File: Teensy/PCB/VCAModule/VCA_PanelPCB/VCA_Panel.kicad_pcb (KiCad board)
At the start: 2 copper layers, 55.9 x 128 mm, 21 parts

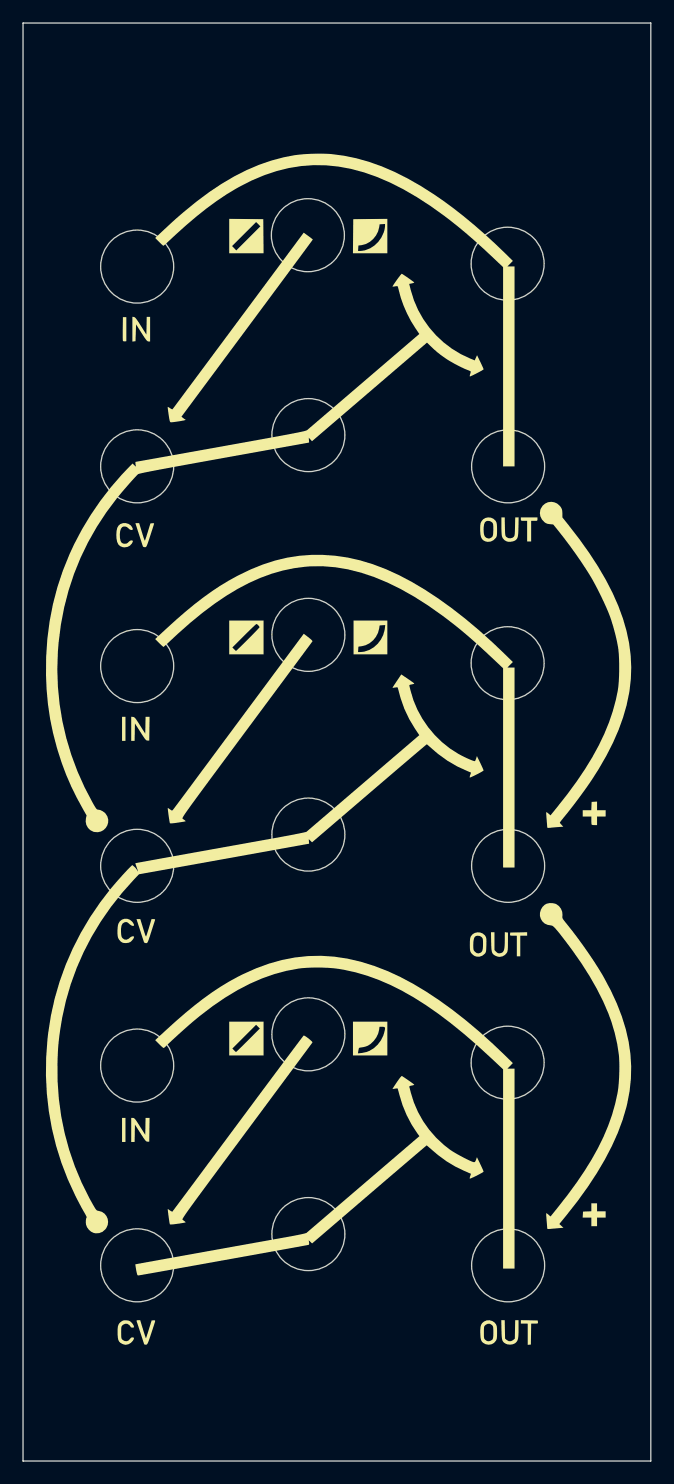
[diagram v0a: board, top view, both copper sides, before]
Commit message: Generated Gerbers
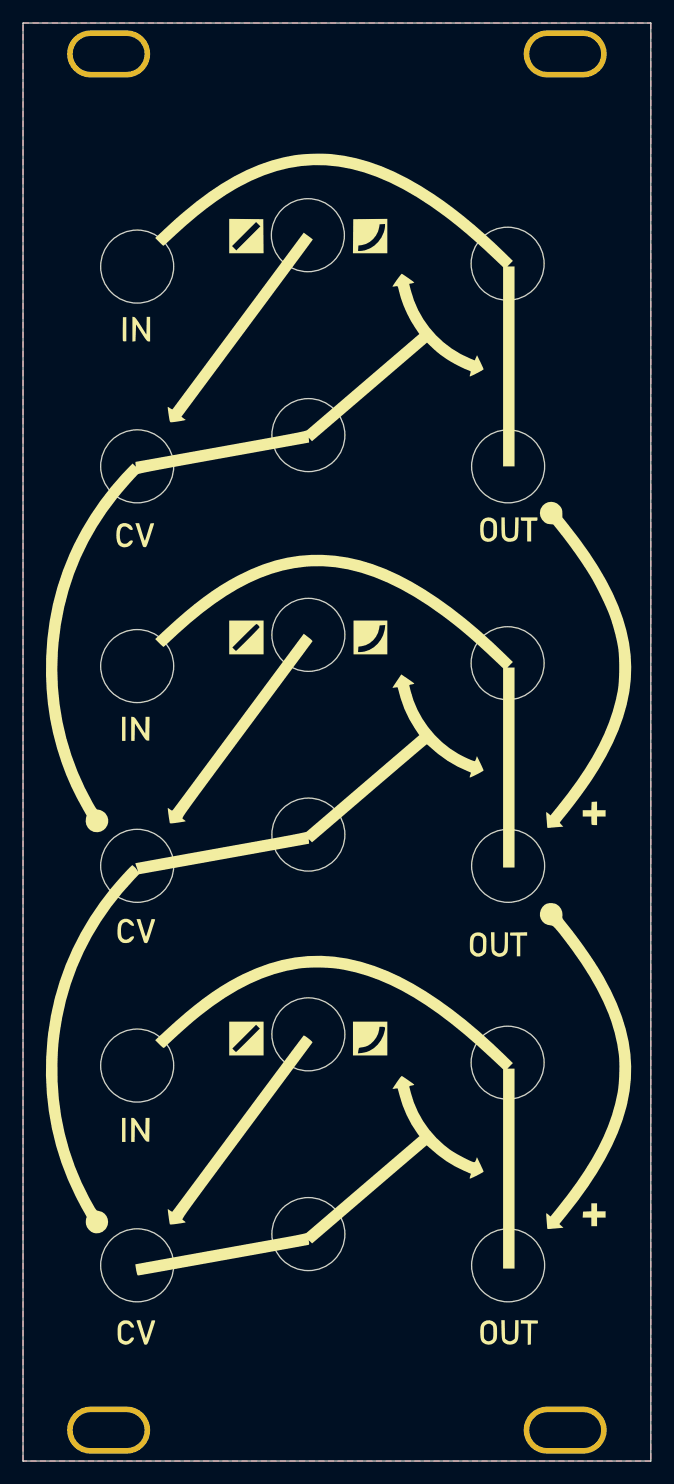
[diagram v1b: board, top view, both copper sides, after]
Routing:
- added copper zone on B.Cu, net shielding
- added copper zone on F.Cu, net shielding
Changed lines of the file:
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@@
       (layerselection 0x00010fc_ffffffff)
       (disableapertmacros false)
-      (usegerberextensions false)
-      (usegerberattributes true)
-      (usegerberadvancedattributes true)
-      (creategerberjobfile true)
+      (usegerberextensions true)
+      (usegerberattributes false)
+      (usegerberadvancedattributes false)
+      (creategerberjobfile false)
       (svguseinch false)
       (svgprecision 6)
@@
       (psa4output false)
       (plotreference true)
-      (plotvalue true)
+      (plotvalue false)
       (plotinvisibletext false)
       (sketchpadsonfab false)
-      (subtractmaskfromsilk false)
+      (subtractmaskfromsilk true)
       (outputformat 1)
       (mirror false)
-      (drillshape 1)
+      (drillshape 0)
       (scaleselection 1)
-      (outputdirectory "")
+      (outputdirectory "VCA_Panel_Gerber")
     )
   )
   (net 0 "")
+  (net 1 "shielding")
   (footprint "Perfboard:3.5mm Jack Perfboard_Hole" (layer "F.Cu")
     (at 114.3 160.02)
@@
     (fp_line (start -2.54 -64) (end 2.54 -64) (layer "User.1") (width 0.12))
     (fp_circle (center 0 0) (end 0 0) (layer "User.1") (width 0.12) (fill none))
-    (fp_line (start -1.27 59.65) (end 1.27 59.65) (layer "User.2") (width 0.12))
-    (fp_line (start -1.27 62.85) (end 1.27 62.85) (layer "User.2") (width 0.12))
-    (fp_line (start -1.27 -62.85) (end 1.27 -62.85) (layer "User.2") (width 0.12))
-    (fp_line (start -1.27 -59.65) (end 1.27 -59.65) (layer "User.2") (width 0.12))
-    (fp_arc (start 1.27 -62.85) (mid 2.87 -61.25) (end 1.27 -59.65) (layer "User.2") (width 0.12))
-    (fp_arc (start -1.27 -59.65) (mid -2.87 -61.25) (end -1.27 -62.85) (layer "User.2") (width 0.12))
-    (fp_arc (start 1.27 59.65) (mid 2.87 61.25) (end 1.27 62.85) (layer "User.2") (width 0.12))
-    (fp_arc (start -1.27 62.85) (mid -2.87 61.25) (end -1.27 59.65) (layer "User.2") (width 0.12))
-    (pad "" np_thru_hole oval (at 0 -61.25) (size 5.74 3.2) (drill oval 5.74 3.2) (layers *.Mask))
-    (pad "" np_thru_hole oval (at 0 61.25) (size 5.74 3.2) (drill oval 5.74 3.2) (layers *.Mask))
+    (fp_line (start -1.6 -62.85) (end 1.6 -62.85) (layer "User.2") (width 0.12))
+    (fp_line (start -1.6 62.85) (end 1.6 62.85) (layer "User.2") (width 0.12))
+    (fp_line (start -1.6 -59.65) (end 1.6 -59.65) (layer "User.2") (width 0.12))
+    (fp_line (start -1.6 59.65) (end 1.6 59.65) (layer "User.2") (width 0.12))
+    (fp_arc (start 1.6 -62.85) (mid 3.2 -61.25) (end 1.6 -59.65) (layer "User.2") (width 0.12))
+    (fp_arc (start -1.6 -59.65) (mid -3.2 -61.25) (end -1.6 -62.85) (layer "User.2") (width 0.12))
+    (fp_arc (start -1.6 62.85) (mid -3.2 61.25) (end -1.6 59.65) (layer "User.2") (width 0.12))
+    (fp_arc (start 1.6 59.65) (mid 3.2 61.25) (end 1.6 62.85) (layer "User.2") (width 0.12))
+    (pad "1" thru_hole oval (at 0 -61.25) (size 7.4 4.2) (drill oval 6.4 3.2) (layers *.Cu *.Mask)
+      (net 1 "shielding"))
+    (pad "1" thru_hole oval (at 0 61.25) (size 7.4 4.2) (drill oval 6.4 3.2) (layers *.Cu *.Mask)
+      (net 1 "shielding"))
   )
   (footprint "Potentiometer:Bourns_PTV09A-XF_Hole" (layer "F.Cu")
@@
     (fp_line (start -2.54 64) (end 2.54 64) (layer "User.1") (width 0.12))
     (fp_circle (center 0 0) (end 0 0) (layer "User.1") (width 0.12) (fill none))
-    (fp_line (start -1.27 -59.65) (end 1.27 -59.65) (layer "User.2") (width 0.12))
-    (fp_line (start -1.27 62.85) (end 1.27 62.85) (layer "User.2") (width 0.12))
-    (fp_line (start -1.27 -62.85) (end 1.27 -62.85) (layer "User.2") (width 0.12))
-    (fp_line (start -1.27 59.65) (end 1.27 59.65) (layer "User.2") (width 0.12))
-    (fp_arc (start 1.27 59.65) (mid 2.87 61.25) (end 1.27 62.85) (layer "User.2") (width 0.12))
-    (fp_arc (start -1.27 62.85) (mid -2.87 61.25) (end -1.27 59.65) (layer "User.2") (width 0.12))
-    (fp_arc (start 1.27 -62.85) (mid 2.87 -61.25) (end 1.27 -59.65) (layer "User.2") (width 0.12))
-    (fp_arc (start -1.27 -59.65) (mid -2.87 -61.25) (end -1.27 -62.85) (layer "User.2") (width 0.12))
-    (pad "" np_thru_hole oval (at 0 61.25) (size 5.74 3.2) (drill oval 5.74 3.2) (layers *.Mask))
-    (pad "" np_thru_hole oval (at 0 -61.25) (size 5.74 3.2) (drill oval 5.74 3.2) (layers *.Mask))
+    (fp_line (start -1.6 59.65) (end 1.6 59.65) (layer "User.2") (width 0.12))
+    (fp_line (start -1.6 -59.65) (end 1.6 -59.65) (layer "User.2") (width 0.12))
+    (fp_line (start -1.6 -62.85) (end 1.6 -62.85) (layer "User.2") (width 0.12))
+    (fp_line (start -1.6 62.85) (end 1.6 62.85) (layer "User.2") (width 0.12))
+    (fp_arc (start 1.6 59.65) (mid 3.2 61.25) (end 1.6 62.85) (layer "User.2") (width 0.12))
+    (fp_arc (start -1.6 62.85) (mid -3.2 61.25) (end -1.6 59.65) (layer "User.2") (width 0.12))
+    (fp_arc (start 1.6 -62.85) (mid 3.2 -61.25) (end 1.6 -59.65) (layer "User.2") (width 0.12))
+    (fp_arc (start -1.6 -59.65) (mid -3.2 -61.25) (end -1.6 -62.85) (layer "User.2") (width 0.12))
+    (pad "1" thru_hole oval (at 0 -61.25) (size 7.4 4.2) (drill oval 6.4 3.2) (layers *.Cu *.Mask)
+      (net 1 "shielding"))
+    (pad "1" thru_hole oval (at 0 61.25) (size 7.4 4.2) (drill oval 6.4 3.2) (layers *.Cu *.Mask)
+      (net 1 "shielding"))
   )
   (footprint "Potentiometer:Bourns_PTV09A-XF_Hole" (layer "F.Cu")
@@
   )
   (gr_rect (start 71.12 50.3) (end 127 178.3) (layer "Edge.Cuts") (width 0.1) (fill none))
+  (zone (net 1) (net_name "shielding") (layers F&B.Cu) (hatch edge 0.508)
+    (connect_pads yes (clearance 0.508))
+    (min_thickness 0.254) (filled_areas_thickness no)
+    (fill yes (thermal_gap 0.508) (thermal_bridge_width 0.508))
+    (polygon
+      (pts
+        (xy 127 178.308)
+        (xy 71.12 178.308)
+        (xy 71.12 50.292)
+        (xy 127 50.292)
+      )
+    )
+  )
 )
